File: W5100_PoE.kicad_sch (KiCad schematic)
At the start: 72 parts, among them J2 ARJM11C7-114-BA-EW2, T1 FA2805, U3 W5100S, U4 TLV431DBZ, U5 VO615A, U6 SI3402, Y2 25MHz

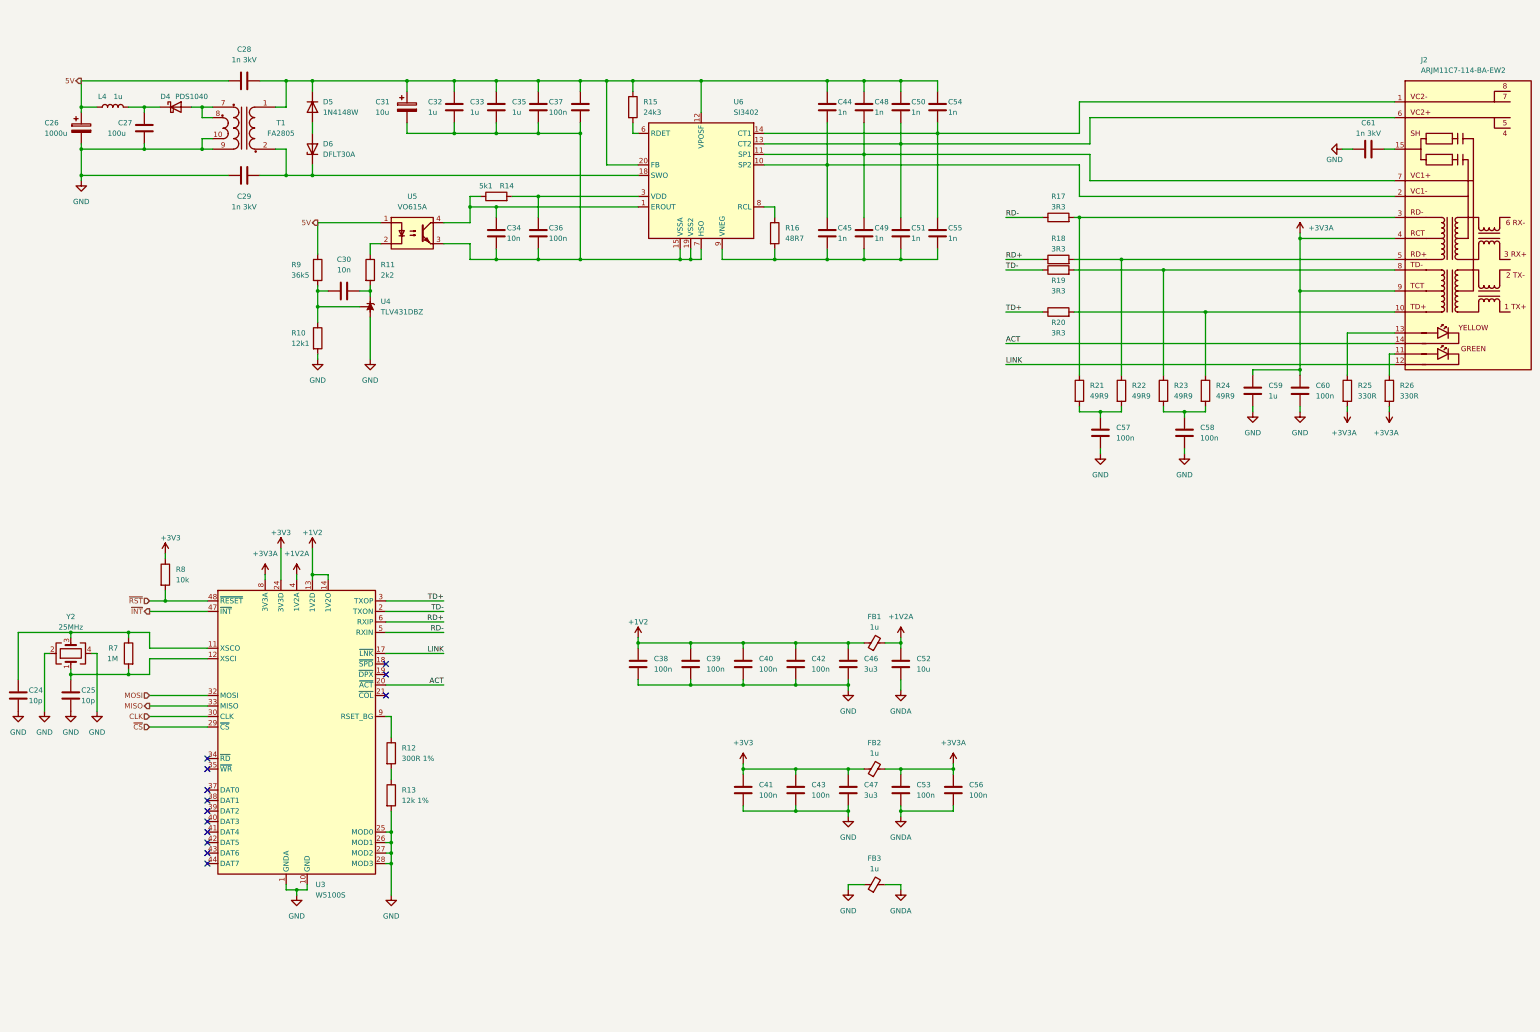
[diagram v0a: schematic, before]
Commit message: Polished schematic
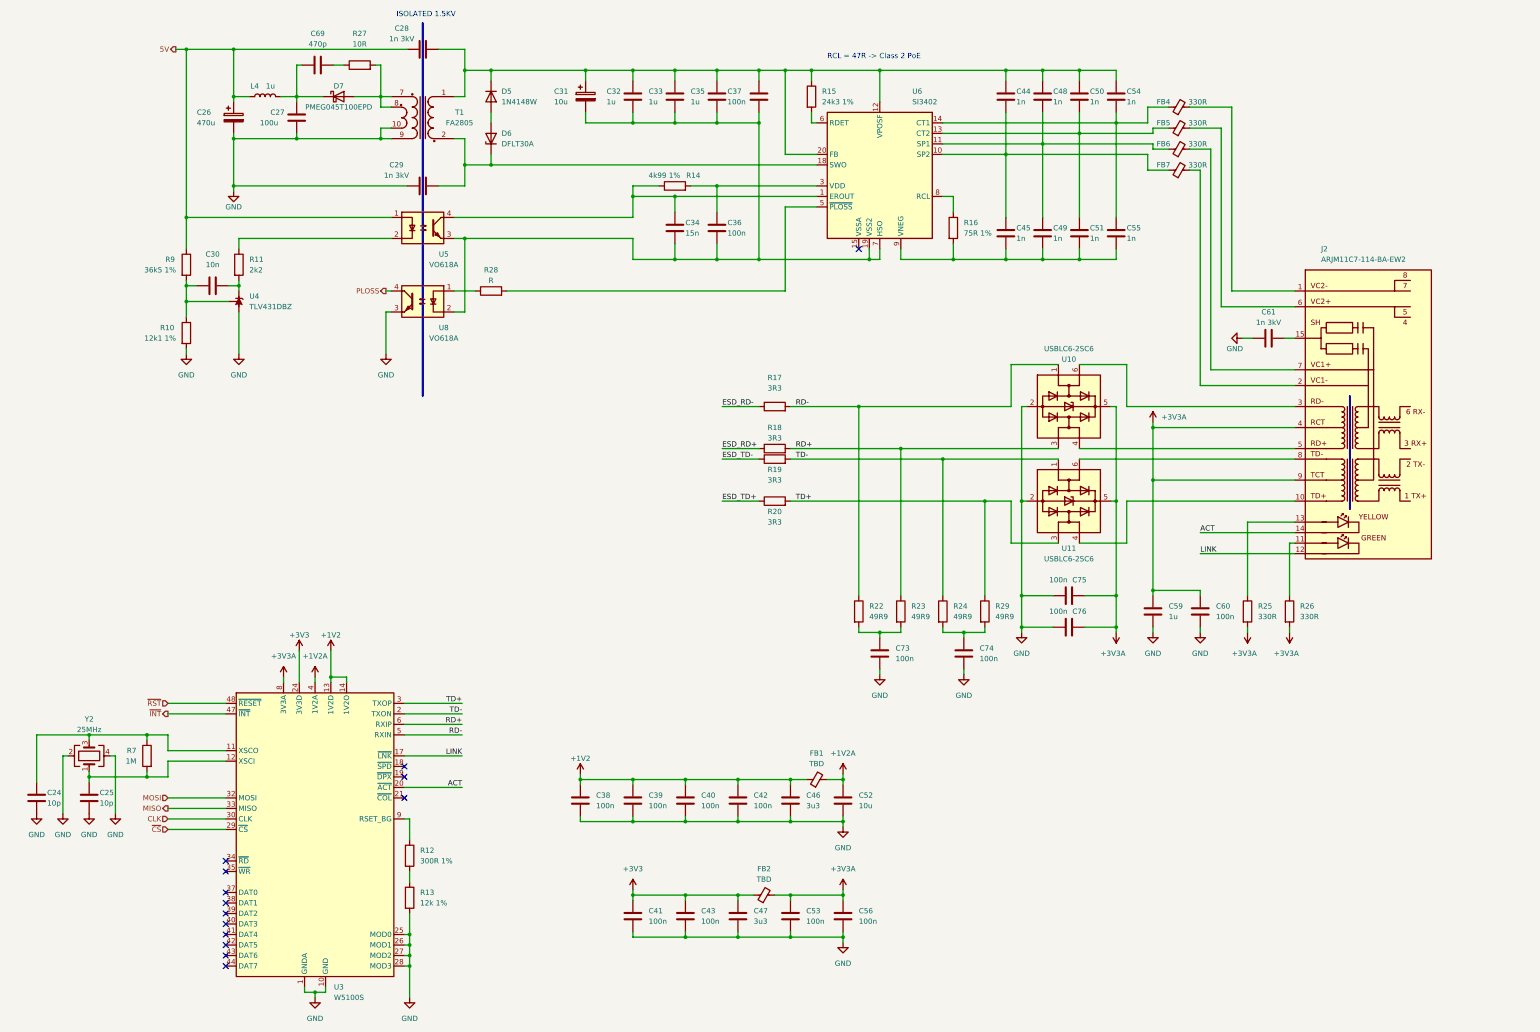
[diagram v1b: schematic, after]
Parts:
- removed C57, C58: 100n, Capacitor_SMD:C_0402_1005Metric, symbol Device:C
- removed D4: PDS1040, symbol Device:D_Schottky
- removed FB3: 1u, Capacitor_SMD:C_0402_1005Metric, symbol Device:FerriteBead_Small
- removed R21: 49R9, Resistor_SMD:R_0402_1005Metric, symbol Device:R
- removed R8: 10k, Resistor_SMD:R_0402_1005Metric, symbol Device:R
- added C69: 470p, Capacitor_SMD:C_0402_1005Metric, symbol Device:C
- added C73, C74, C75, C76: 100n, Capacitor_SMD:C_0402_1005Metric, symbol Device:C
- added D7: PMEG045T100EPD, Package_TO_SOT_SMD:Nexperia_CFP15_SOT-1289, symbol Diode:PMEG045T100EPD
- added FB4, FB5, FB6, FB7: 330R, Inductor_SMD:L_0805_2012Metric, symbol Device:FerriteBead_Small
- added R27: 10R, Resistor_SMD:R_0402_1005Metric, symbol Device:R
- added R28: R, Resistor_SMD:R_0402_1005Metric, symbol Device:R
- added R29: 49R9, Resistor_SMD:R_0402_1005Metric, symbol Device:R
- added U10, U11: USBLC6-2SC6, Package_TO_SOT_SMD:SOT-23-6, symbol Power_Protection:USBLC6-2SC6
- added U8: VO618A, Package_SO:SO-4_7.6x3.6mm_P2.54mm, symbol Isolator:VO615A
- C26: value 1000u -> 470u; footprint (none) -> Capacitor_Tantalum_SMD:CP_EIA-2012-12_Kemet-R
- C27, C28, C29, C61: footprint (none) -> Capacitor_SMD:C_1206_3216Metric
- C32, C33, C35, C59, L4: footprint Capacitor_SMD:C_0402_1005Metric -> Capacitor_SMD:C_0603_1608Metric
- C34: value 10n -> 15n
- C46, C47, C52: footprint (none) -> Capacitor_SMD:C_0603_1608Metric
- D6: footprint (none) -> Diode_SMD:D_PowerDI-123
- FB1, FB2: value 1u -> TBD
- J2: footprint (none) -> abracon:ARJM11C7-114-BA-EW2
- R10: value 12k1 -> 12k1 1%
- R14: value 5k1 -> 4k99 1%
- R15: value 24k3 -> 24k3 1%
- R16: value 48R7 -> 75R 1%
- R9: value 36k5 -> 36k5 1%
- U5: value VO615A -> VO618A; footprint (none) -> Package_SO:SO-4_7.6x3.6mm_P2.54mm
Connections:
- net GNDA is gone; now on net GND: C52.2, C53.2, C56.2
- net +3V3A: now also C75.2, C76.2, U10.5 (VBUS), U11.5 (VBUS)
- net GND: now also C73.2, C74.2, C75.1, C76.1, U10.2 (GND), U11.2 (GND), U8.3
- net RD+: now also R18.2, R23.1, U10.3 (I/O2); no longer R18.1
- net RD-: now also R17.2, R22.1, U10.1 (I/O1); no longer R17.1
- net TD+: now also R20.2, R29.1, U11.3 (I/O2); no longer R20.1
- net TD-: now also R19.2, R24.1, U11.1 (I/O1); no longer R19.1
- net at R23.2: now also R22.2, C73.1; no longer R24.2
- net at T1.7, T1.8: now also D7.1 (A), D7.2 (A), R27.2
- net at C54.2, C55.1, U6.14 (CT1): now also FB4.1; no longer J2.1
- net at C44.2, C45.1, U6.10 (SP2): now also FB7.1; no longer J2.2
- net at J2.3: now also U10.6 (I/O1); no longer R17.2
- net at C50.2, C51.1, U6.13 (CT2): now also FB5.1; no longer J2.6
- net at C48.2, C49.1, U6.11 (SP1): now also FB6.1; no longer J2.7
- net at C31.2, C32.2, C33.2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: now also U8.2; no longer U6.15 (VSSA)
- net at C27.1, L4.2: now also C69.1, D7.3 (K)
- new net: FB4.2, J2.1
- new net: J2.10, U11.4 (I/O2)
- new net: FB7.2, J2.2
- new net: J2.5, U10.4 (I/O2)
- new net: FB5.2, J2.6
- new net: FB6.2, J2.7
- new net: J2.8, U11.6 (I/O1)
- new net: R28.2, U6.5 (~{PLOSS})
- new net: C74.1, R24.2, R29.2
- new net: R28.1, U8.1
- new net: C69.2, R27.1
- new net ESD_RD+: R18.1
- new net ESD_RD-: R17.1
- new net ESD_TD+: R20.1
- new net ESD_TD-: R19.1
- new net PLOSS: U8.4
- no-connect marks 13 -> 14
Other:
- note added: "ISOLATED 1.5KV"
- note added: "RCL = 47R -> Class 2 PoE"
- moved on the sheet: C24, C25, C26, C27, C28, C29, C30, C31, C32, C33, C34, C35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
